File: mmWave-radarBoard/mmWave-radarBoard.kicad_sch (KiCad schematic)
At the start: 4 parts

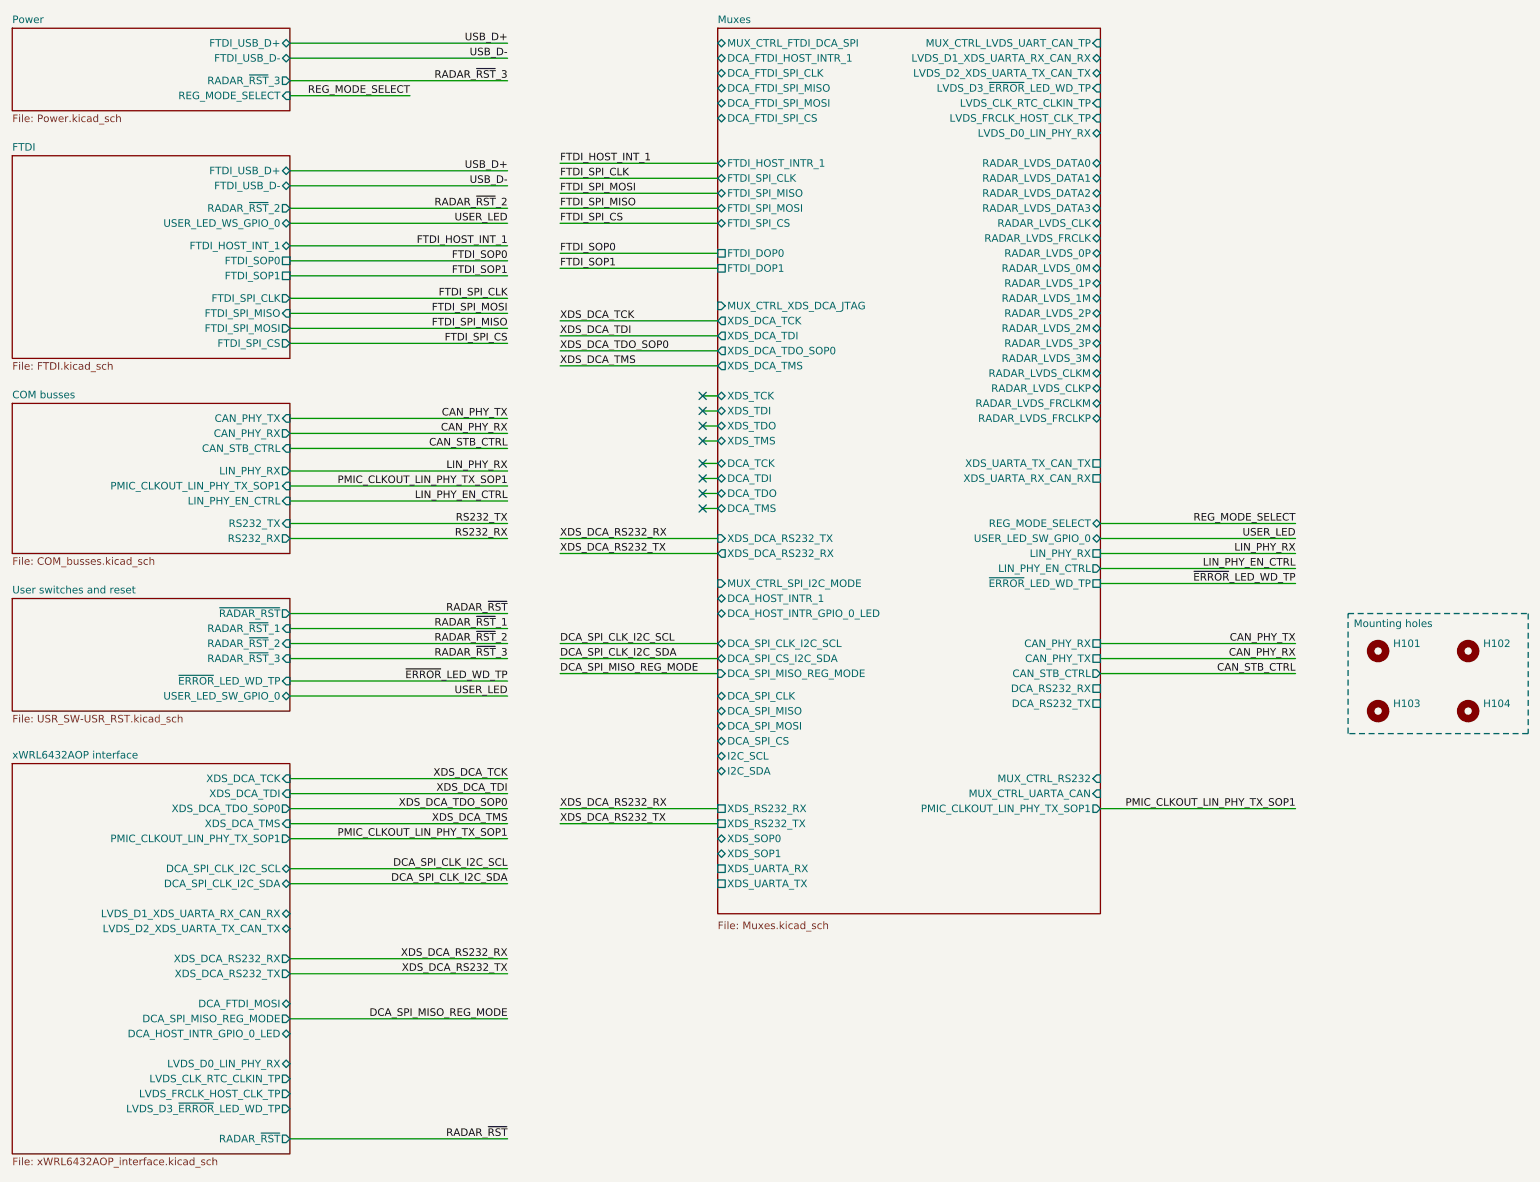
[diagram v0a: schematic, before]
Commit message: Removed unnecessary bits
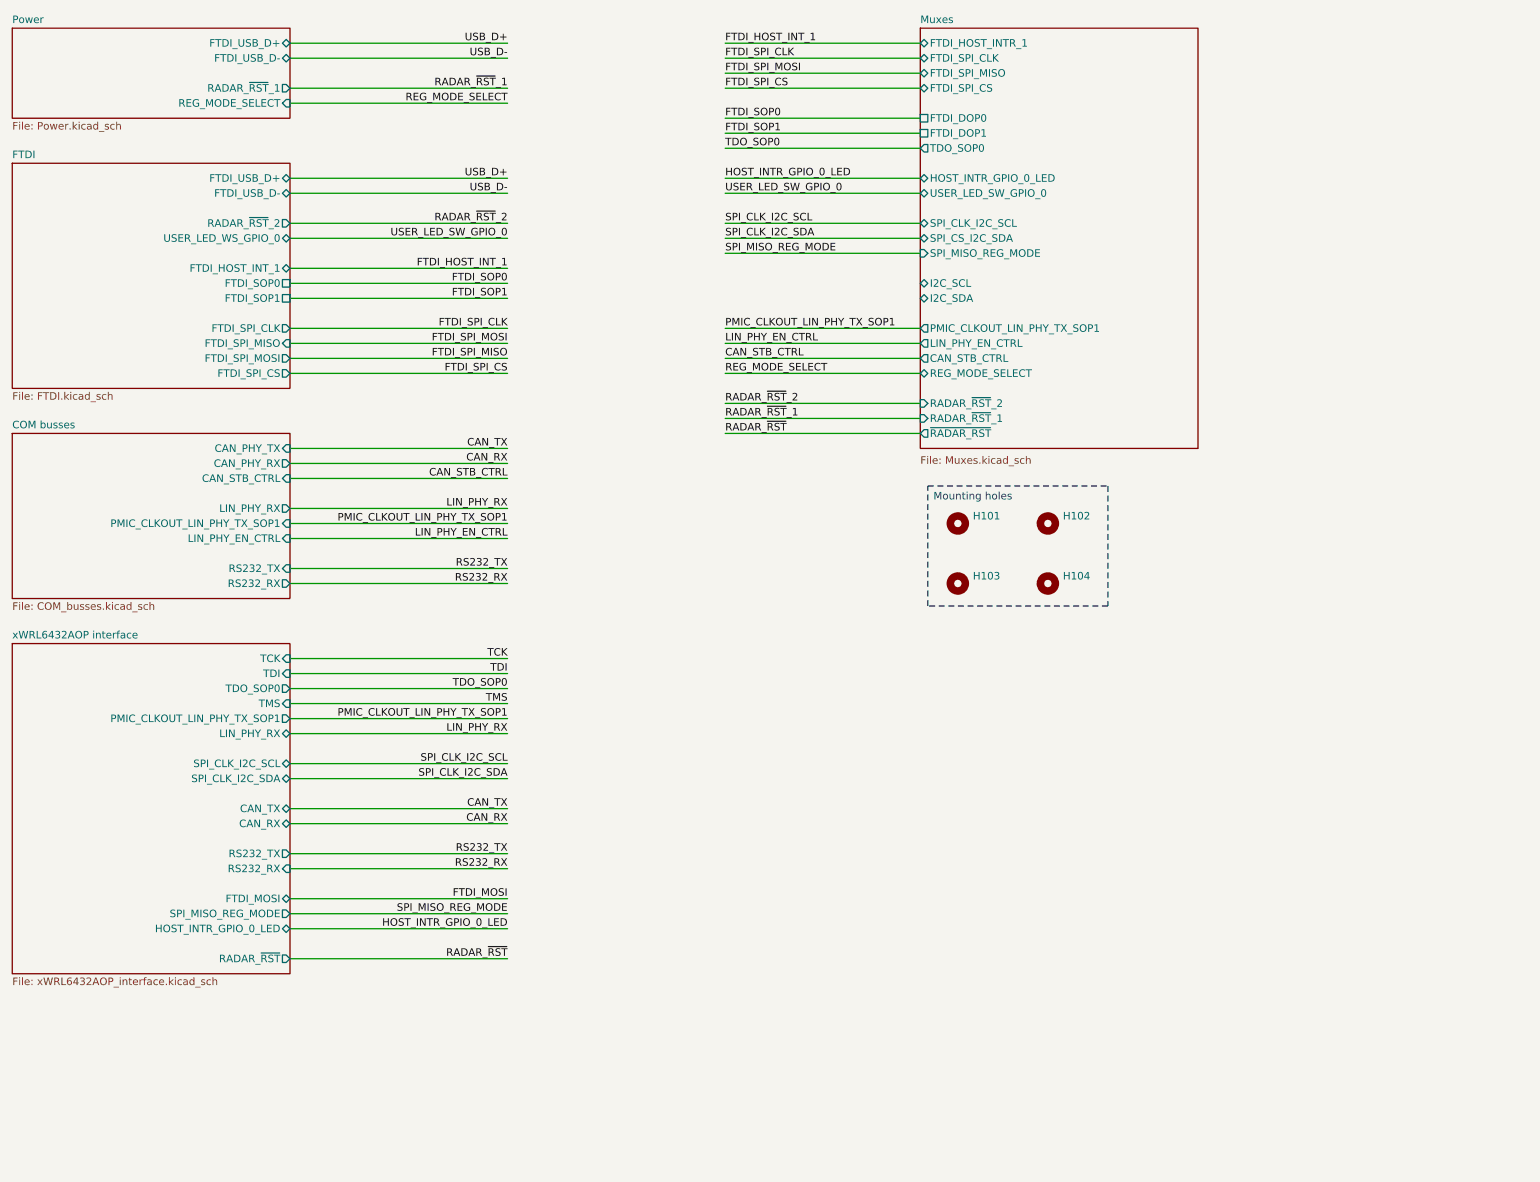
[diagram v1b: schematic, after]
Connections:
- no-connect marks 8 -> 0
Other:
- removed sheet User switches and reset
- sheet Muxes ports: added HOST_INTR_GPIO_0_LED, RADAR_~{RST}_1, RADAR_~{RST}_2, SPI_CLK_I2C_SCL, SPI_CS_I2C_SDA, SPI_MISO_REG_MODE, TDO_SOP0, ~{RADAR_RST}; removed CAN_PHY_RX, CAN_PHY_TX, DCA_FTDI_HOST_INTR_1, DCA_FTDI_SPI_CLK, DCA_FTDI_SPI_CS, DCA_FTDI_SPI_MISO, DCA_FTDI_SPI_MOSI, DCA_HOST_INTR_1, DCA_HOST_INTR_GPIO_0_LED, DCA_RS232_RX, DCA_RS232_TX, DCA_SPI_CLK, DCA_SPI_CLK_I2C_SCL, DCA_SPI_CS, DCA_SPI_CS_I2C_SDA, DCA_SPI_MISO, DCA_SPI_MISO_REG_MODE, DCA_SPI_MOSI, DCA_TCK, DCA_TDI, DCA_TDO, DCA_TMS, FTDI_SPI_MOSI, LIN_PHY_RX, LVDS_CLK_RTC_CLKIN_TP, LVDS_D0_LIN_PHY_RX, LVDS_D1_XDS_UARTA_RX_CAN_RX, LVDS_D2_XDS_UARTA_TX_CAN_TX, LVDS_D3_~{ERROR}_LED_WD_TP, LVDS_FRCLK_HOST_CLK_TP, MUX_CTRL_FTDI_DCA_SPI, MUX_CTRL_LVDS_UART_CAN_TP, MUX_CTRL_RS232, MUX_CTRL_SPI_I2C_MODE, MUX_CTRL_UARTA_CAN, MUX_CTRL_XDS_DCA_JTAG, RADAR_LVDS_0M, RADAR_LVDS_0P, RADAR_LVDS_1M, RADAR_LVDS_1P, RADAR_LVDS_2M, RADAR_LVDS_2P, RADAR_LVDS_3M, RADAR_LVDS_3P, RADAR_LVDS_CLK, RADAR_LVDS_CLKM, RADAR_LVDS_CLKP, RADAR_LVDS_DATA0, RADAR_LVDS_DATA1, RADAR_LVDS_DATA2, RADAR_LVDS_DATA3, RADAR_LVDS_FRCLK, RADAR_LVDS_FRCLKM, RADAR_LVDS_FRCLKP, XDS_DCA_RS232_RX, XDS_DCA_RS232_TX, XDS_DCA_TCK, XDS_DCA_TDI, XDS_DCA_TDO_SOP0, XDS_DCA_TMS, XDS_RS232_RX, XDS_RS232_TX, XDS_SOP0, XDS_SOP1, XDS_TCK, XDS_TDI, XDS_TDO, XDS_TMS, XDS_UARTA_RX, XDS_UARTA_RX_CAN_RX, XDS_UARTA_TX, XDS_UARTA_TX_CAN_TX, ~{ERROR}_LED_WD_TP
- sheet Power ports: added RADAR_~{RST}_1; removed RADAR_~{RST}_3
- sheet xWRL6432AOP interface ports: added CAN_RX, CAN_TX, FTDI_MOSI, HOST_INTR_GPIO_0_LED, LIN_PHY_RX, RS232_RX, RS232_TX, SPI_CLK_I2C_SCL, SPI_CLK_I2C_SDA, SPI_MISO_REG_MODE, TCK, TDI, TDO_SOP0, TMS; removed DCA_FTDI_MOSI, DCA_HOST_INTR_GPIO_0_LED, DCA_SPI_CLK_I2C_SCL, DCA_SPI_CLK_I2C_SDA, DCA_SPI_MISO_REG_MODE, LVDS_CLK_RTC_CLKIN_TP, LVDS_D0_LIN_PHY_RX, LVDS_D1_XDS_UARTA_RX_CAN_RX, LVDS_D2_XDS_UARTA_TX_CAN_TX, LVDS_D3_~{ERROR}_LED_WD_TP, LVDS_FRCLK_HOST_CLK_TP, XDS_DCA_RS232_RX, XDS_DCA_RS232_TX, XDS_DCA_TCK, XDS_DCA_TDI, XDS_DCA_TDO_SOP0, XDS_DCA_TMS
- moved on the sheet: H101, H102, H103, H104
